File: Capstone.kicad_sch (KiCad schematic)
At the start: 4 parts, among them J2 Conn_01x08_Socket, U1 XIAO-ESP32-S3-DIP, U11 SN74HC161DR, U3 74LS151

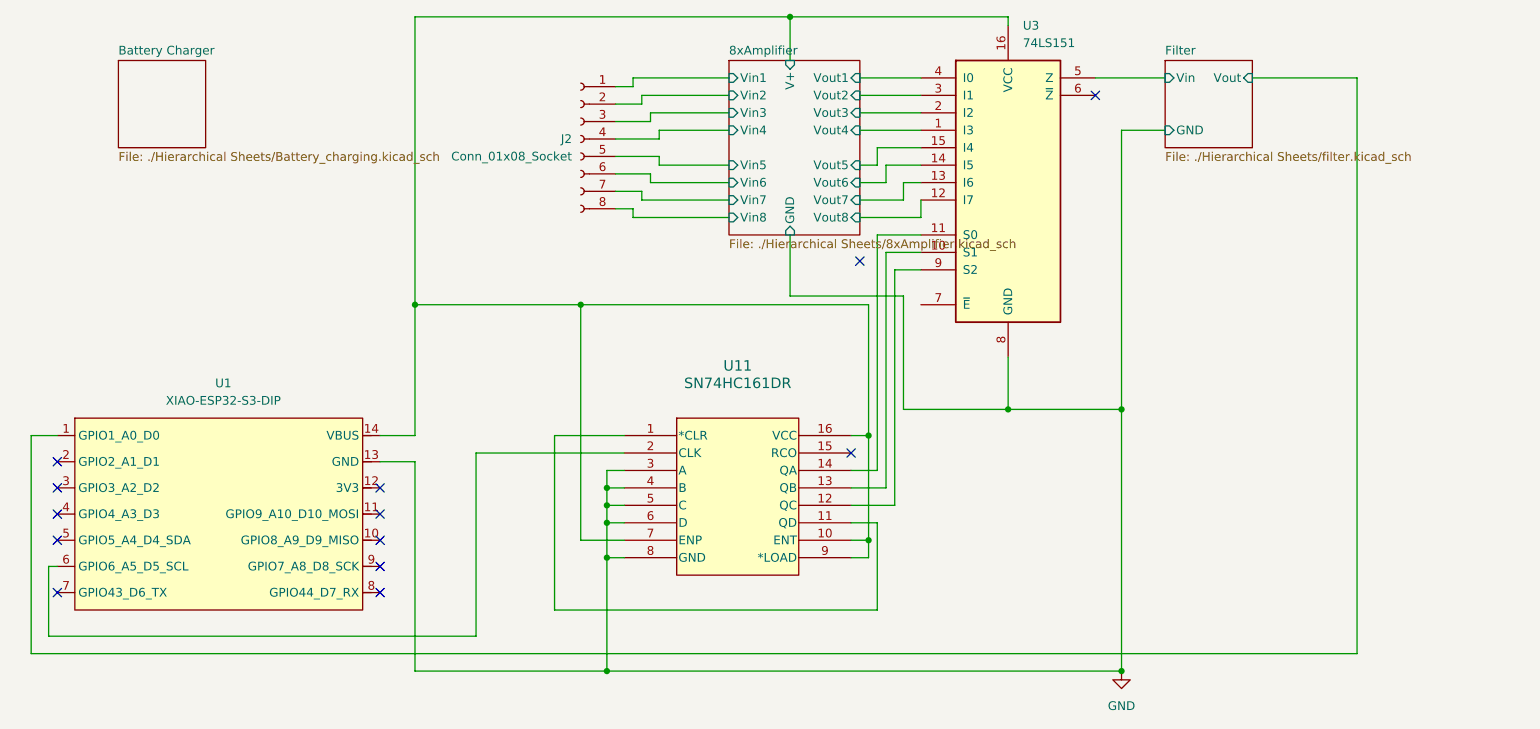
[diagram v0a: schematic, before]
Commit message: Redo Base Project file add code
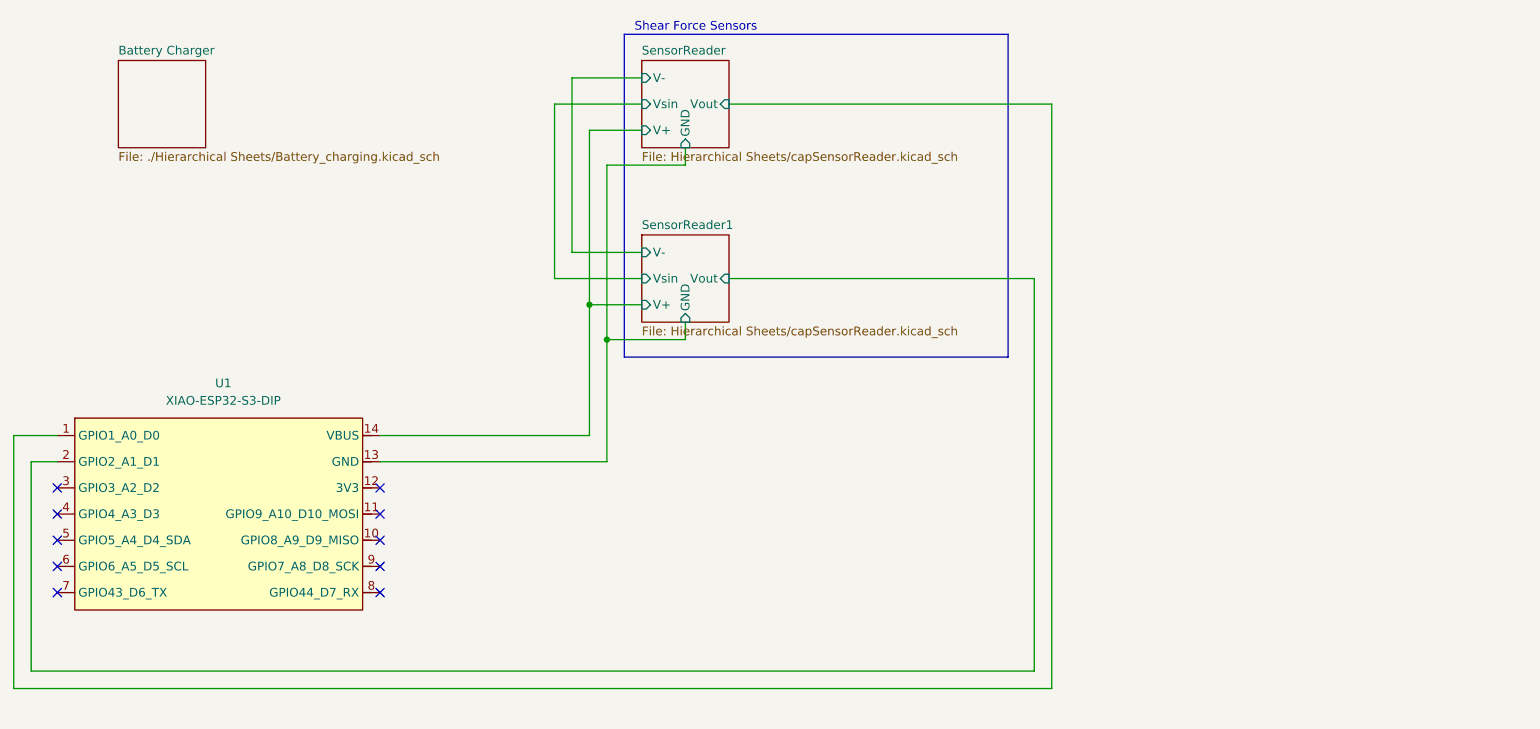
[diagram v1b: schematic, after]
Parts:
- removed J2: Conn_01x08_Socket, symbol Connector:Conn_01x08_Socket
- removed U11: SN74HC161DR, CapstoneFootprints:D16, symbol Capstone:SN74HC161DR
- removed U3: 74LS151, CapstoneFootprints:D16, symbol 74xx:74LS151
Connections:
- net SensorReader1/Vout: now reaches U1.2 (GPIO2_A1_D1)
- net 8xAmplifier/V+ renamed SensorReader/V+
- net Filter/Vout renamed SensorReader/Vout
- net GND renamed SensorReader/GND
- no-connect marks 13 -> 10
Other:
- removed sheet 8xAmplifier
- removed sheet Filter
- added sheet SensorReader (Hierarchical Sheets/capSensorReader.kicad_sch)
- added sheet SensorReader1 (Hierarchical Sheets/capSensorReader.kicad_sch)
- note added: "Shear Force Sensors"
